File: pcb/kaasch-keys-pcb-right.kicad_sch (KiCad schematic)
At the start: 73 parts, among them J1 Conn_01x12_Pin, J2 Conn_01x12_Pin, SW1 SW_Push, SW10 SW_Push, SW11 SW_Push, SW12 SW_Push, SW13 SW_Push, SW14 SW_Push, SW15 SW_Push, SW16 SW_Push, SW17 SW_Push, SW18 SW_Push, SW19 SW_Push, SW2 SW_Push, SW20 SW_Push, SW21 SW_Push, SW22 SW_Push, SW23 SW_Push, SW24 SW_Push, SW25 SW_Push, SW26 SW_Push, SW27 SW_Push, SW28 SW_Push, SW29 SW_Push, SW3 SW_Push, SW30 SW_Push, SW31 SW_Push, SW32 SW_Push, SW33 SW_Push, SW34 SW_Push, SW35 SW_Push, SW36 SW_Push_Reset, SW4 SW_Push, SW5 SW_Push, SW6 SW_Push, SW7 SW_Push, SW8 SW_Push, SW9 SW_Push

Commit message: swaggers
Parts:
- SW10, SW4: footprint Button_Switch_Keyboard:SW_Cherry_MX_1.00u_PCB -> Button_Switch_Keyboard:SW_Cherry_MX_1.50u_PCB
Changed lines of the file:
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@@
 			)
 		)
-		(property "Footprint" "Button_Switch_Keyboard:SW_Cherry_MX_1.00u_PCB"
+		(property "Footprint" "Button_Switch_Keyboard:SW_Cherry_MX_1.50u_PCB"
 			(at 223.52 119.38 0)
 			(effects
@@
 			)
 		)
-		(property "Footprint" "Button_Switch_Keyboard:SW_Cherry_MX_1.00u_PCB"
+		(property "Footprint" "Button_Switch_Keyboard:SW_Cherry_MX_1.50u_PCB"
 			(at 246.38 101.6 0)
 			(effects

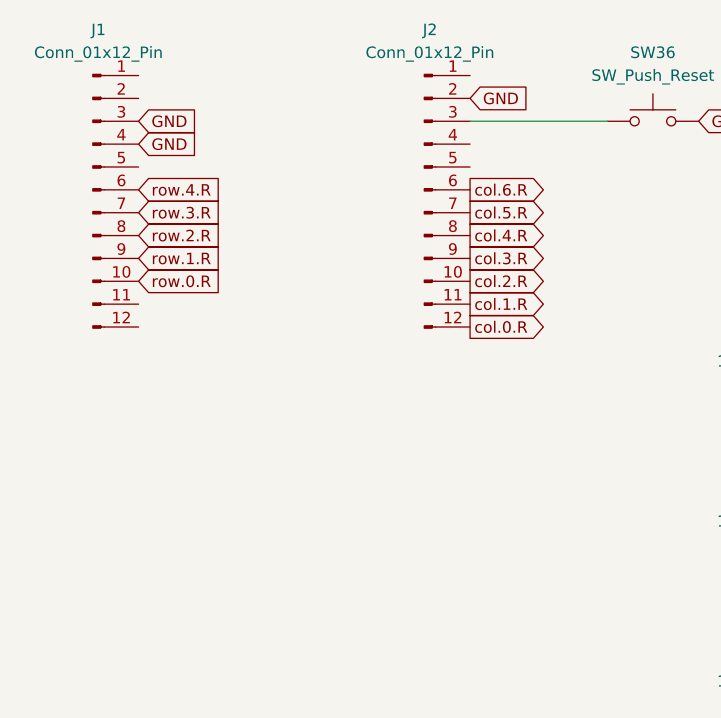
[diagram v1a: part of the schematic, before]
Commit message: continue on design
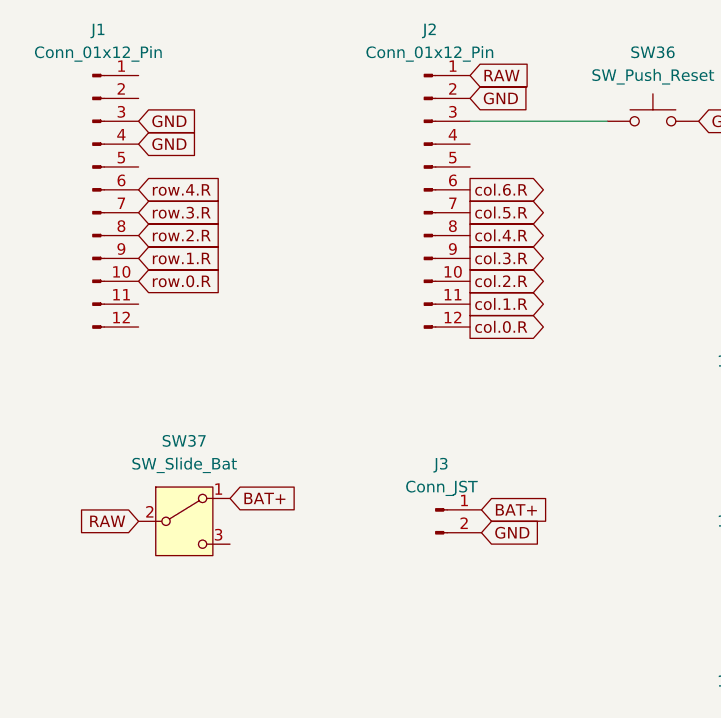
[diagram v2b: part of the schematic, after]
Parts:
- added J3: Conn_JST, Connector_JST:JST_EH_B2B-EH-A_1x02_P2.50mm_Vertical, symbol Connector:Conn_01x02_Pin
- added SW37: SW_Slide_Bat, Button_Switch_SMD:SW_SPDT_PCM12, symbol Switch:SW_SPDT
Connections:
- net GND: now also J3.2 (Pin_2)
- net RAW: now reaches J2.1 (Pin_1)
- net RAW: now also SW37.2 (B)
- new net BAT+: J3.1 (Pin_1), SW37.1 (A)
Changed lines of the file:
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@@
 		)
 	)
+	(global_label "GND"
+		(shape input)
+		(at 68.58 77.47 0)
+		(fields_autoplaced yes)
+		(effects
+			(font
+				(size 1.27 1.27)
+			)
+			(justify left)
+		)
+		(property "Intersheetrefs" "${INTERSHEET_REFS}"
+			(at 75.4357 77.47 0)
+			(effects
+				(font
+					(size 1.27 1.27)
+				)
+				(justify left)
+				(hide yes)
+			)
+		)
+	)
 	(global_label "col.2.R"
 		(shape output)
@@
 		)
 	)
+	(global_label "RAW"
+		(shape input)
+		(at 67.31 26.67 0)
+		(fields_autoplaced yes)
+		(effects
+			(font
+				(size 1.27 1.27)
+			)
+			(justify left)
+		)
+		(property "Intersheetrefs" "${INTERSHEET_REFS}"
+			(at 74.1052 26.67 0)
+			(effects
+				(font
+					(size 1.27 1.27)
+				)
+				(justify left)
+				(hide yes)
+			)
+		)
+	)
 	(global_label "col.3.R"
 		(shape input)
@@
 		)
 	)
+	(global_label "BAT+"
+		(shape input)
+		(at 40.64 73.66 0)
+		(fields_autoplaced yes)
+		(effects
+			(font
+				(size 1.27 1.27)
+			)
+			(justify left)
+		)
+		(property "Intersheetrefs" "${INTERSHEET_REFS}"
+			(at 48.5238 73.66 0)
+			(effects
+				(font
+					(size 1.27 1.27)
+				)
+				(justify left)
+				(hide yes)
+			)
+		)
+	)
 	(global_label "col.0.R"
 		(shape input)
@@
 		)
 	)
+	(global_label "BAT+"
+		(shape input)
+		(at 68.58 74.93 0)
+		(fields_autoplaced yes)
+		(effects
+			(font
+				(size 1.27 1.27)
+			)
+			(justify left)
+		)
+		(property "Intersheetrefs" "${INTERSHEET_REFS}"
+			(at 76.4638 74.93 0)
+			(effects
+				(font
+					(size 1.27 1.27)
+				)
+				(justify left)
+				(hide yes)
+			)
+		)
+	)
 	(global_label "GND"
 		(shape input)
@@
 		)
 	)
+	(global_label "RAW"
+		(shape input)
+		(at 30.48 76.2 180)
+		(fields_autoplaced yes)
+		(effects
+			(font
+				(size 1.27 1.27)
+			)
+			(justify right)
+		)
+		(property "Intersheetrefs" "${INTERSHEET_REFS}"
+			(at 23.6848 76.2 0)
+			(effects
+				(font
+					(size 1.27 1.27)
+				)
+				(justify right)
+				(hide yes)
+			)
+		)
+	)
 	(global_label "col.6.R"
 		(shape output)
@@
 	)
 	(symbol
+		(lib_id "Connector:Conn_01x02_Pin")
+		(at 63.5 74.93 0)
+		(unit 1)
+		(exclude_from_sim no)
+		(in_bom yes)
+		(on_board yes)
+		(dnp no)
+		(fields_autoplaced yes)
+		(property "Reference" "J3"
+			(at 64.135 69.85 0)
+			(effects
+				(font
+					(size 1.27 1.27)
+				)
+			)
+		)
+		(property "Value" "Conn_JST"
+			(at 64.135 72.39 0)
+			(effects
+				(font
+					(size 1.27 1.27)
+				)
+			)
+		)
+		(property "Footprint" "Connector_JST:JST_EH_B2B-EH-A_1x02_P2.50mm_Vertical"
+			(at 63.5 74.93 0)
+			(effects
+				(font
+					(size 1.27 1.27)
+				)
+				(hide yes)
+			)
+		)
+		(property "Datasheet" "~"
+			(at 63.5 74.93 0)
+			(effects
+				(font
+					(size 1.27 1.27)
+				)
+				(hide yes)
+			)
+		)
+		(property "Description" "Generic connector, single row, 01x02, script generated"
+			(at 63.5 74.93 0)
+			(effects
+				(font
+					(size 1.27 1.27)
+				)
+				(hide yes)
+			)
+		)
+		(pin "1"
+		)
+		(pin "2"
+		)
+		(instances
+			(project "kaasch-keys-pcb-right"
+				(path "/5acf686b-48cf-4069-a41d-20ff58a52189"
+					(reference "J3")
+					(unit 1)
+				)
+			)
+		)
+	)
+	(symbol
 		(lib_id "Diode:1N4148")
 		(at 78.74 140.97 270)
@@
 					(unit 1)
 				)
+			)
+		)
+	)
+	(symbol
+		(lib_id "Switch:SW_SPDT")
+		(at 35.56 76.2 0)
+		(unit 1)
+		(exclude_from_sim no)
+		(in_bom yes)
+		(on_board yes)
+		(dnp no)
+		(fields_autoplaced yes)
+		(property "Reference" "SW37"
+			(at 35.56 67.31 0)
+			(effects
+				(font
+					(size 1.27 1.27)
+				)
+			)
+		)
+		(property "Value" "SW_Slide_Bat"
+			(at 35.56 69.85 0)
+			(effects
+				(font
+					(size 1.27 1.27)
+				)
+			)
+		)
+		(property "Footprint" "Button_Switch_SMD:SW_SPDT_PCM12"
+			(at 35.56 76.2 0)
+			(effects
+				(font
+					(size 1.27 1.27)
+				)
+				(hide yes)
+			)
+		)
+		(property "Datasheet" "~"
+			(at 35.56 83.82 0)
+			(effects
+				(font
+					(size 1.27 1.27)
+				)
+				(hide yes)
+			)
+		)
+		(property "Description" "Switch, single pole double throw"
+			(at 35.56 76.2 0)
+			(effects
+				(font
+					(size 1.27 1.27)
+				)
+				(hide yes)
+			)
+		)
+		(pin "1"
+		)
+		(pin "3"
+		)
+		(pin "2"
+		)
+		(instances
+			(project "kaasch-keys-pcb-right"
+				(path "/5acf686b-48cf-4069-a41d-20ff58a52189"
+					(reference "SW37")
+					(unit 1)
+				)
